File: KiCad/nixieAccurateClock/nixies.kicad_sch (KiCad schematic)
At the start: 0 parts

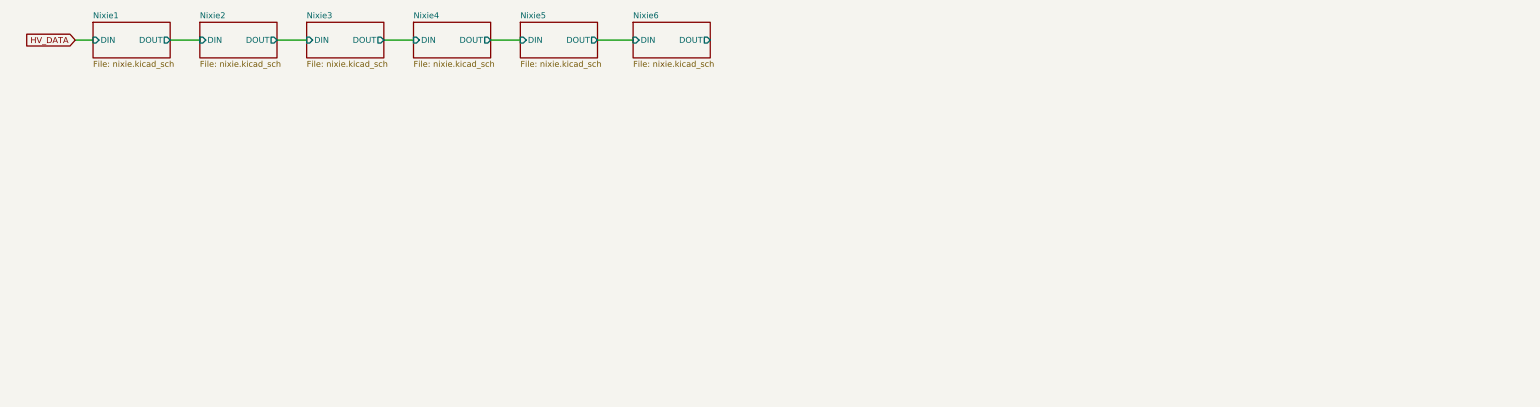
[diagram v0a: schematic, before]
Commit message: IN-14 daughter board
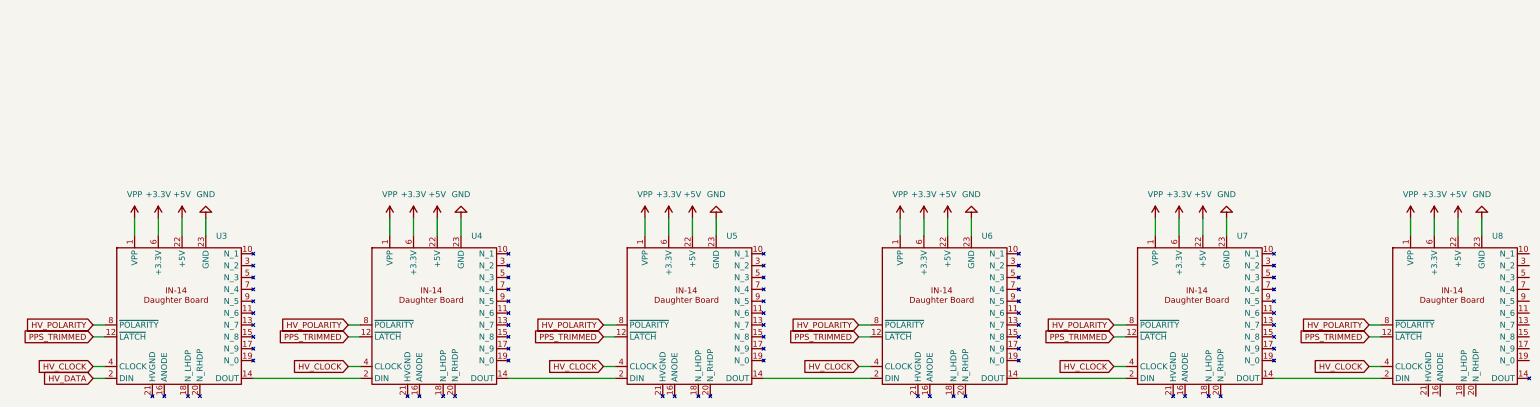
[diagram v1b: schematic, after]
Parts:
- added U3, U4, U5, U6, U7, U8: ~, 00_lib:IN-14 daughter board, symbol 00_lib:IN-14_daughter_board
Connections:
- net HV_DATA: now also U3.2 (DIN)
- new net: U5.14 (DOUT), U6.2 (DIN)
- new net: U4.14 (DOUT), U5.2 (DIN)
- new net: U7.14 (DOUT), U8.2 (DIN)
- new net: U6.14 (DOUT), U7.2 (DIN)
- new net: U3.14 (DOUT), U4.2 (DIN)
- new net +3.3V: U3.6 (+3.3V), U4.6 (+3.3V), U5.6 (+3.3V), U6.6 (+3.3V), U7.6 (+3.3V), U8.6 (+3.3V)
- new net +5V: U3.22 (+5V), U4.22 (+5V), U5.22 (+5V), U6.22 (+5V), U7.22 (+5V), U8.22 (+5V)
- new net GND: U3.23 (GND), U4.23 (GND), U5.23 (GND), U6.23 (GND), U7.23 (GND), U8.23 (GND)
- new net HV_CLOCK: U3.4 (CLOCK), U4.4 (CLOCK), U5.4 (CLOCK), U6.4 (CLOCK), U7.4 (CLOCK), U8.4 (CLOCK)
- new net HV_POLARITY: U3.8 (~{POLARITY}), U4.8 (~{POLARITY}), U5.8 (~{POLARITY}), U6.8 (~{POLARITY}), U7.8 (~{POLARITY}), U8.8 (~{POLARITY})
- new net PPS_TRIMMED: U3.12 (~{LATCH}), U4.12 (~{LATCH}), U5.12 (~{LATCH}), U6.12 (~{LATCH}), U7.12 (~{LATCH}), U8.12 (~{LATCH})
- new net VPP: U3.1 (VPP), U4.1 (VPP), U5.1 (VPP), U6.1 (VPP), U7.1 (VPP), U8.1 (VPP)
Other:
- removed sheet Nixie1
- removed sheet Nixie2
- removed sheet Nixie3
- removed sheet Nixie4
- removed sheet Nixie5
- removed sheet Nixie6
